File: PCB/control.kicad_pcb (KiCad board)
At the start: 2 copper layers, 86 x 50 mm, 9 parts, among them P1 CONN_01X07, P13 CONN_01X07, P14 CONN_01X04, P5 BATTERY, P8 CONN_01X04, U1 4056_CARG

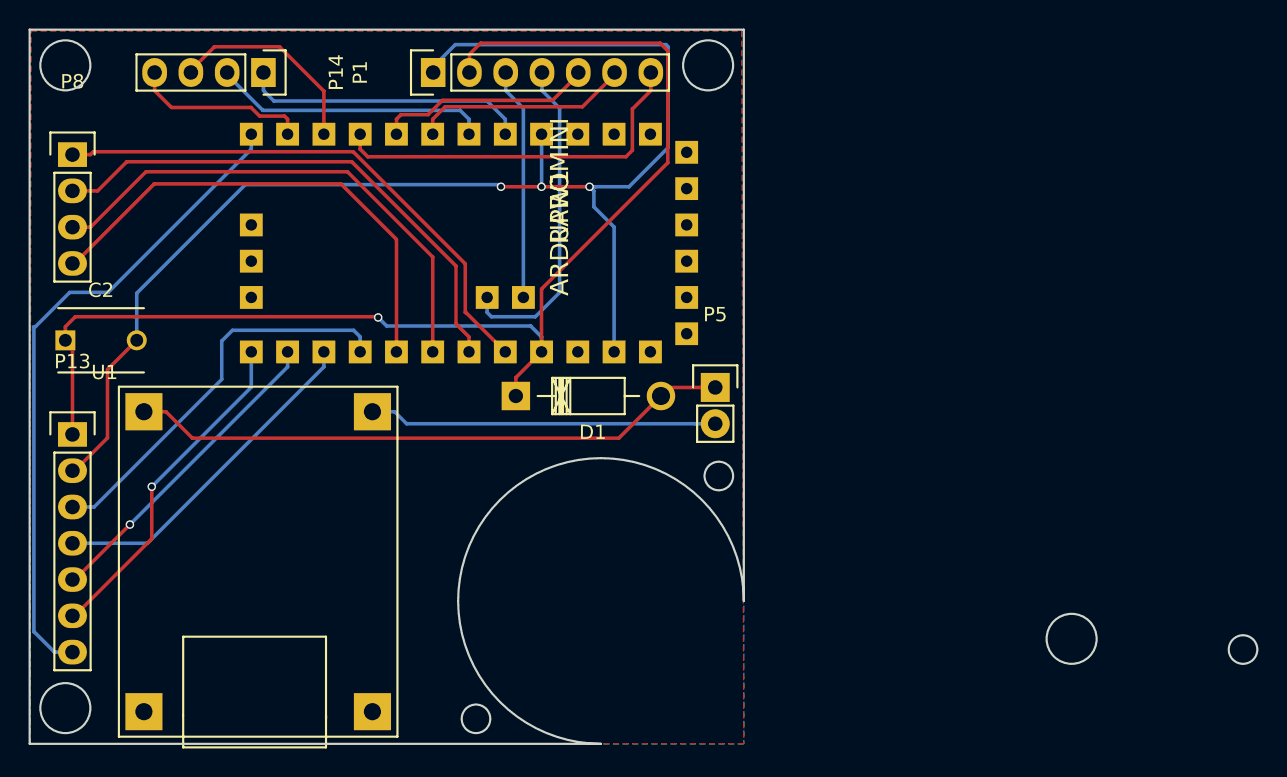
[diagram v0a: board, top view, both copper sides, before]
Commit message: Fix PCBs
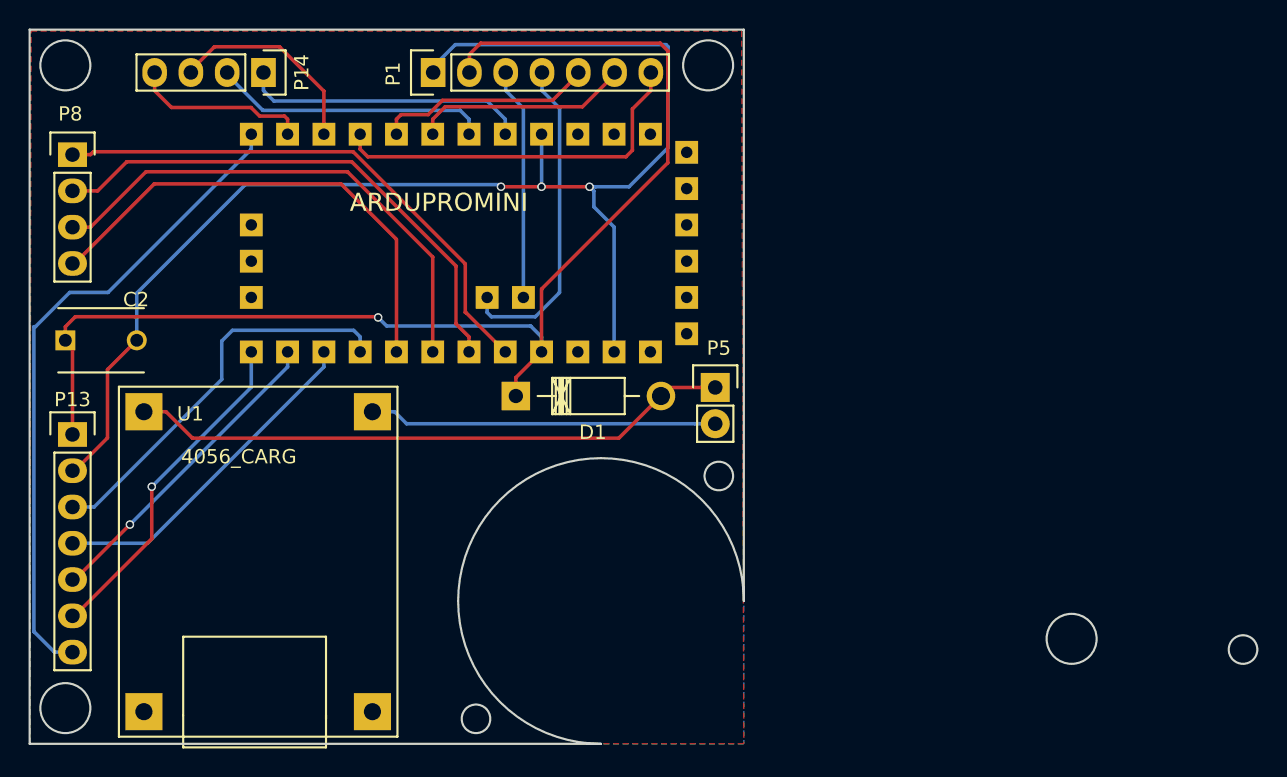
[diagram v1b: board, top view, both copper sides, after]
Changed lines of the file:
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@@
-(kicad_pcb (version 4) (host pcbnew 4.0.0-rc1-stable)
+(kicad_pcb (version 4) (host pcbnew 4.0.2+dfsg1-stable)
   (general
     (links 29)
-    (no_connects 2)
-    (area 37.351725 28.448816 278.178572 182.950001)
+    (no_connects 0)
+    (area 84.474999 53.824999 170.575001 103.975001)
     (thickness 1.6)
     (drawings 32)
@@
   (module 4056_lipoCharg (layer F.Cu)
     (at 89.8 77.4)
-    (fp_text reference U1 (at 0 0.5) (layer F.SilkS)
-      (effects (font (size 1 1) (thickness 0.15)))
-    )
-    (fp_text value 4056_CARG (at 0 -0.5) (layer F.Fab)
+    (fp_text reference U1 (at 6 3.4) (layer F.SilkS)
+      (effects (font (size 1 1) (thickness 0.15)))
+    )
+    (fp_text value 4056_CARG (at 9.4 6.4) (layer F.SilkS)
       (effects (font (size 1 1) (thickness 0.15)))
     )
@@
     (at 121.66 66.3 270)
     (descr ABK-PRO-MINI)
-    (fp_text reference RAW1 (at 0 0 270) (layer F.SilkS)
+    (fp_text reference RAW1 (at 2.9 10.86 360) (layer F.Fab)
       (effects (font (thickness 0.15)))
     )
-    (fp_text value ARDUPROMINI (at 0 0 270) (layer F.SilkS)
+    (fp_text value ARDUPROMINI (at -0.3 8.46 360) (layer F.SilkS)
       (effects (font (thickness 0.15)))
     )
@@
     (descr "Through hole pin header")
     (tags "pin header")
-    (fp_text reference P1 (at 0 -5.1 90) (layer F.SilkS)
+    (fp_text reference P1 (at -0.1 -2.8 90) (layer F.SilkS)
       (effects (font (size 1 1) (thickness 0.15)))
     )
@@
     (descr "Through hole pin header")
     (tags "pin header")
-    (fp_text reference P5 (at 0 -5.1) (layer F.SilkS)
-      (effects (font (size 1 1) (thickness 0.15)))
-    )
-    (fp_text value BATTERY (at 0 -3.1) (layer F.Fab)
+    (fp_text reference P5 (at 0.25 -2.75) (layer F.SilkS)
+      (effects (font (size 1 1) (thickness 0.15)))
+    )
+    (fp_text value BATTERY (at -1.95 3.25 90) (layer F.Fab)
       (effects (font (size 1 1) (thickness 0.15)))
     )
@@
     (descr "Through hole pin header")
     (tags "pin header")
-    (fp_text reference P8 (at 0 -5.1) (layer F.SilkS)
+    (fp_text reference P8 (at -0.15 -2.85) (layer F.SilkS)
       (effects (font (size 1 1) (thickness 0.15)))
     )
@@
     (descr "Through hole pin header")
     (tags "pin header")
-    (fp_text reference P13 (at 0 -5.1) (layer F.SilkS)
+    (fp_text reference P13 (at 0 -2.44) (layer F.SilkS)
       (effects (font (size 1 1) (thickness 0.15)))
     )
@@
     (descr "Through hole pin header")
     (tags "pin header")
-    (fp_text reference P14 (at 0 -5.1 270) (layer F.SilkS)
+    (fp_text reference P14 (at 0 -2.68 270) (layer F.SilkS)
       (effects (font (size 1 1) (thickness 0.15)))
     )
@@
     (descr "Capacitor 6mm Disc, Pitch 5mm")
     (tags Capacitor)
-    (fp_text reference C2 (at 2.5 -3.5) (layer F.SilkS)
+    (fp_text reference C2 (at 4.95 -2.85) (layer F.SilkS)
       (effects (font (size 1 1) (thickness 0.15)))
     )
@@
   (segment (start 129.1 54.95) (end 129.25 55.1) (width 0.25) (layer B.Cu) (net 1))
   (segment (start 114.35 54.95) (end 129.1 54.95) (width 0.25) (layer B.Cu) (net 1))
-  (segment (start 112.8 56.5) (end 114.35 54.95) (width 0.25) (layer B.Cu) (net 1) (status 400000))
-  (segment (start 112.8 56.9) (end 112.8 56.5) (width 0.25) (layer B.Cu) (net 1) (status C00000))
+  (segment (start 112.8 56.5) (end 114.35 54.95) (width 0.25) (layer B.Cu) (net 1))
+  (segment (start 112.8 56.9) (end 112.8 56.5) (width 0.25) (layer B.Cu) (net 1))
   (segment (start 90 82.4824) (end 90 77.7) (width 0.25) (layer F.Cu) (net 1))
   (segment (start 90 77.7) (end 92.05 75.65) (width 0.25) (layer F.Cu) (net 1))
